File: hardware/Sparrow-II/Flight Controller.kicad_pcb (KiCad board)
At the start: 4 copper layers, 42 x 42 mm, 4 parts

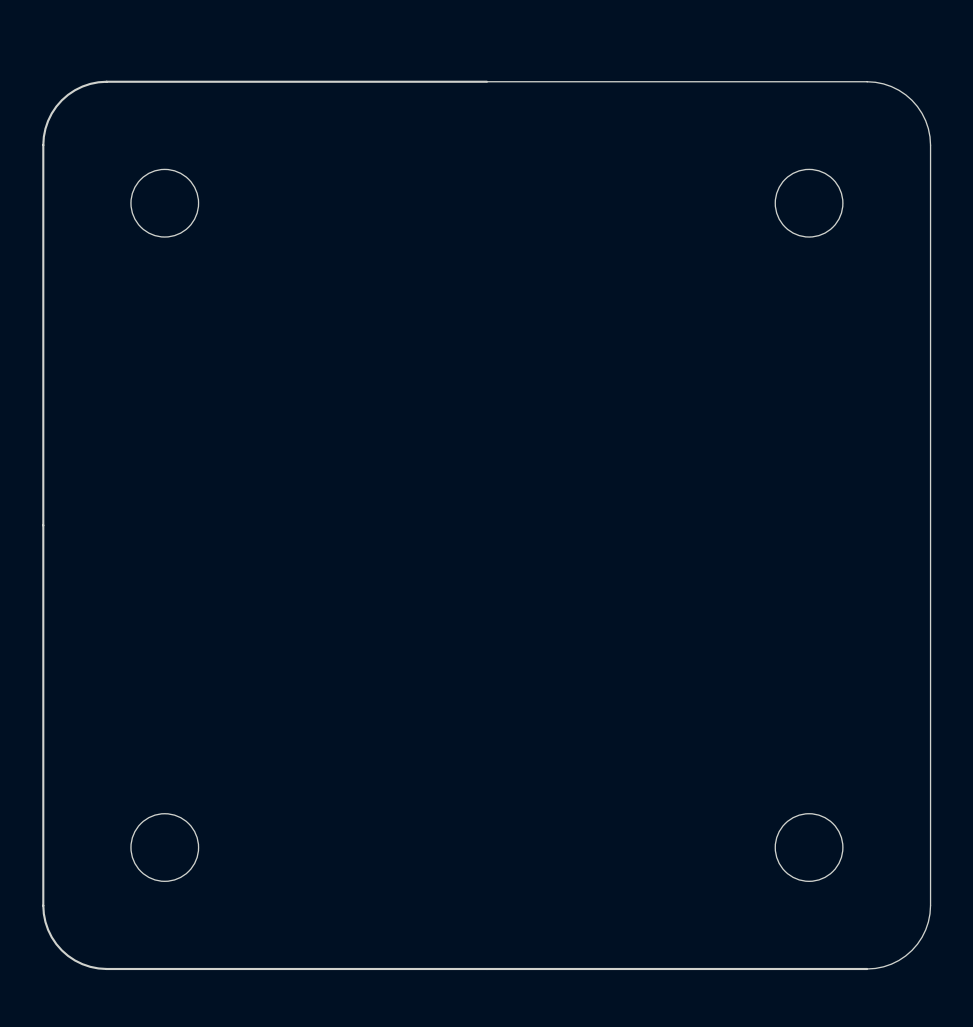
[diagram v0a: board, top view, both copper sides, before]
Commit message: hardware: first layout and optimalizations
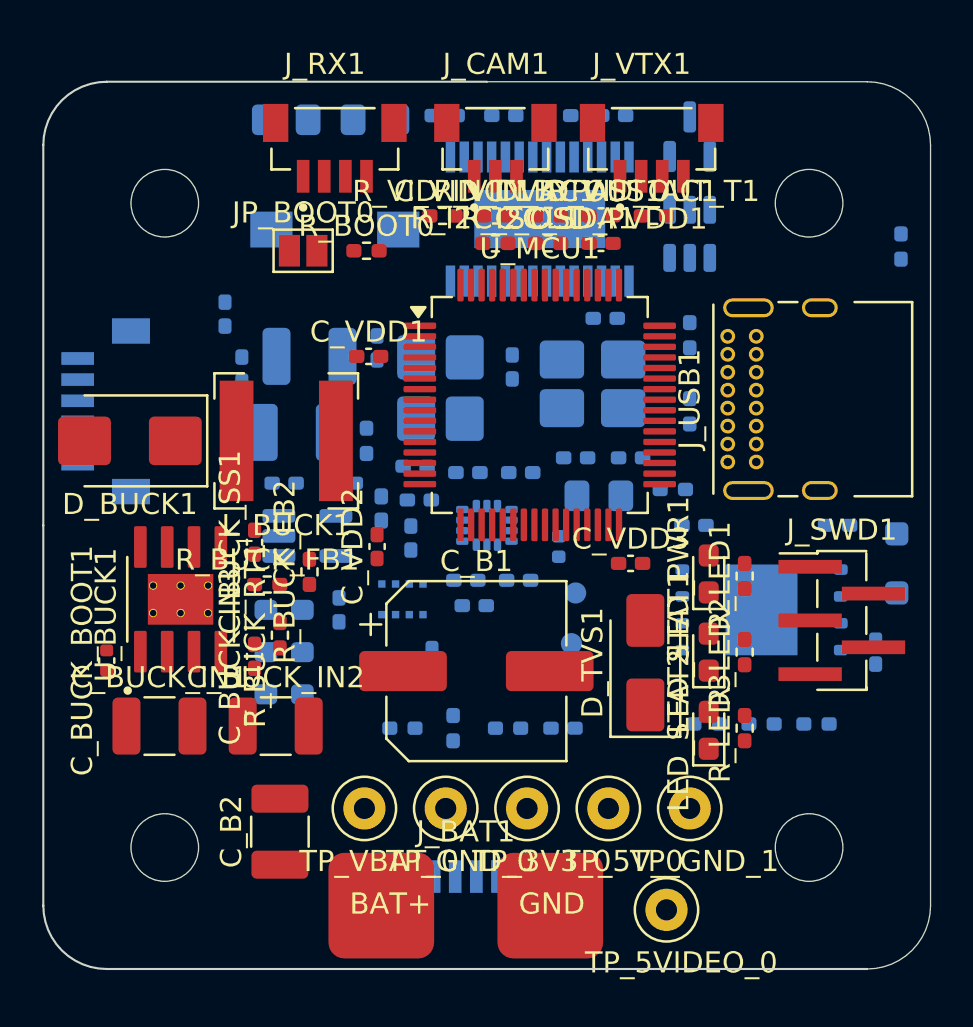
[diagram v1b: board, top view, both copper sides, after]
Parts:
- added C_3V3_BULK1: 10uF, Capacitor_SMD:C_0603_1608Metric_Pad1.08x0.95mm_HandSolder, B.Cu at (140.4, 104.0)
- added C_5V_BULK1: 10uF, Capacitor_SMD:C_0603_1608Metric_Pad1.08x0.95mm_HandSolder, B.Cu at (140.4, 108.0)
- added C_B1: 470uF, Capacitor_SMD:CP_Elec_8x6.9, F.Cu at (149.5, 106.9)
- added C_B2: 10uF, Capacitor_SMD:C_1210_3225Metric_Pad1.33x2.70mm_HandSolder, F.Cu at (140.2, 114.5)
- added C_B3: 1uF, Capacitor_SMD:C_0603_1608Metric_Pad1.08x0.95mm_HandSolder, B.Cu at (140.4, 106.0)
- added C_B4: 100nF, Capacitor_SMD:C_0402_1005Metric_Pad0.74x0.62mm_HandSolder, B.Cu at (143.0, 104.0)
- added C_BARO1: 100nF, Capacitor_SMD:C_0402_1005Metric_Pad0.74x0.62mm_HandSolder, B.Cu at (145.0, 106.4)
- added C_BARO2: 100nF, Capacitor_SMD:C_0402_1005Metric_Pad0.74x0.62mm_HandSolder, B.Cu at (147.4, 106.4)
- added C_BUCK_BOOT1: 100nF, Capacitor_SMD:C_0402_1005Metric, F.Cu at (132.0, 106.4)
- added C_BUCK_IN1: 2.2uF, Capacitor_SMD:C_1210_3225Metric_Pad1.33x2.70mm_HandSolder, F.Cu at (134.5, 109.5)
- added C_BUCK_IN2: 2.2uF, Capacitor_SMD:C_1210_3225Metric_Pad1.33x2.70mm_HandSolder, F.Cu at (140.0, 109.5)
- added C_BUCK_IN3: 100nF, Capacitor_SMD:C_0402_1005Metric_Pad0.74x0.62mm_HandSolder, F.Cu at (139.0, 106.2)
- added C_BUCK_OUT1: 47uF, Capacitor_SMD:C_1210_3225Metric_Pad1.33x2.70mm_HandSolder, B.Cu at (141.6, 92.0)
- added C_BUCK_OUT2: 47uF, Capacitor_SMD:C_1210_3225Metric_Pad1.33x2.70mm_HandSolder, B.Cu at (141.0, 95.6)
- added C_BUCK_SS1: 22nF, Capacitor_SMD:C_0402_1005Metric_Pad0.74x0.62mm_HandSolder, F.Cu at (139.0, 100.8)
- added C_CURR_F1: 1uF, Capacitor_SMD:C_0402_1005Metric_Pad0.74x0.62mm_HandSolder, B.Cu at (153.6, 109.6)
- added C_FLASH1: 100nF, Capacitor_SMD:C_0402_1005Metric_Pad0.74x0.62mm_HandSolder, B.Cu at (168.4, 106.0)
- added C_HSE1: 12pF, Capacitor_SMD:C_0402_1005Metric_Pad0.74x0.62mm_HandSolder, B.Cu at (146.6, 97.2)
- added C_HSE2: 12pF, Capacitor_SMD:C_0402_1005Metric_Pad0.74x0.62mm_HandSolder, B.Cu at (151.2, 92.5)
- added C_IMU_VDD1: 2.2uF, Capacitor_SMD:C_0402_1005Metric_Pad0.74x0.62mm_HandSolder, B.Cu at (151.5, 102.6)
- added C_IMU_VDD2: 100nF, Capacitor_SMD:C_0402_1005Metric_Pad0.74x0.62mm_HandSolder, B.Cu at (151.6, 97.5)
- added C_IMU_VIO1: 100nF, Capacitor_SMD:C_0402_1005Metric_Pad0.74x0.62mm_HandSolder, B.Cu at (149.1, 97.5)
- added C_IMU_VIO2: 10nF, Capacitor_SMD:C_0402_1005Metric_Pad0.74x0.62mm_HandSolder, B.Cu at (149.0, 102.6)
- added C_LDO_IN1: 1uF, Capacitor_SMD:C_0402_1005Metric_Pad0.74x0.62mm_HandSolder, B.Cu at (140.4, 98.0)
- added C_LDO_OUT1: 1uF, Capacitor_SMD:C_0402_1005Metric_Pad0.74x0.62mm_HandSolder, B.Cu at (143.2, 98.0)
- added C_NRST1: 100nF, Capacitor_SMD:C_0402_1005Metric_Pad0.74x0.62mm_HandSolder, B.Cu at (149.4, 103.8)
- added C_OSD_AVDD1: 100nF, Capacitor_SMD:C_0402_1005Metric_Pad0.74x0.62mm_HandSolder, B.Cu at (150.8, 80.6)
- added C_OSD_DVDD1: 100nF, Capacitor_SMD:C_0402_1005Metric_Pad0.74x0.62mm_HandSolder, B.Cu at (155.6, 90.2)
- added C_OSD_PVDD1: 4.7uF, Capacitor_SMD:C_0402_1005Metric_Pad0.74x0.62mm_HandSolder, F.Cu at (155.4, 86.7)
- added C_OSD_PVDD2: 100nF, Capacitor_SMD:C_0402_1005Metric_Pad0.74x0.62mm_HandSolder, B.Cu at (153.4, 80.6)
- added C_OSD_SAG1: 22uF, Capacitor_SMD:C_0402_1005Metric_Pad0.74x0.62mm_HandSolder, B.Cu at (156.0, 80.6)
- added C_OSD_XTAL1: 27pF, Capacitor_SMD:C_0402_1005Metric_Pad0.74x0.62mm_HandSolder, B.Cu at (154.2, 96.8)
- added C_OSD_XTAL2: 27pF, Capacitor_SMD:C_0402_1005Metric_Pad0.74x0.62mm_HandSolder, B.Cu at (156.8, 96.8)
- added C_USB_SH1: 10nF, Capacitor_SMD:C_0402_1005Metric_Pad0.74x0.62mm_HandSolder, B.Cu at (166.6, 100.0)
- added C_VBAT_ADC1: 100nF, Capacitor_SMD:C_0402_1005Metric_Pad0.74x0.62mm_HandSolder, B.Cu at (138.4, 92.6)
- added C_VCAP1: 4.7uF, Capacitor_SMD:C_0805_2012Metric_Pad1.18x1.45mm_HandSolder, B.Cu at (155.3, 98.6)
- added C_VDD1: 100nF, Capacitor_SMD:C_0402_1005Metric_Pad0.74x0.62mm_HandSolder, F.Cu at (144.4, 92.0)
- added C_VDD2: 100nF, Capacitor_SMD:C_0402_1005Metric_Pad0.74x0.62mm_HandSolder, F.Cu at (144.8, 101.0)
- added C_VDD3: 100nF, Capacitor_SMD:C_0402_1005Metric_Pad0.74x0.62mm_HandSolder, F.Cu at (156.8, 101.8)
- added C_VDD4: 100nF, Capacitor_SMD:C_0402_1005Metric_Pad0.74x0.62mm_HandSolder, B.Cu at (159.8, 100.0)
- added C_VDDA1: 1uF, Capacitor_SMD:C_0402_1005Metric_Pad0.74x0.62mm_HandSolder, B.Cu at (146.4, 100.6)
- added C_VDDA_HF1: 100nF, Capacitor_SMD:C_0402_1005Metric_Pad0.74x0.62mm_HandSolder, B.Cu at (146.8, 98.8)
- added C_VDD_BULK1: 4.7uF, Capacitor_SMD:C_0402_1005Metric_Pad0.74x0.62mm_HandSolder, B.Cu at (144.8, 91.6)
- added C_VID1: 22uF, Capacitor_SMD:C_0805_2012Metric_Pad1.18x1.45mm_HandSolder, B.Cu at (140.5, 80.8)
- added C_VID2: 22uF, Capacitor_SMD:C_0805_2012Metric_Pad1.18x1.45mm_HandSolder, B.Cu at (144.7, 80.8)
- added C_VID3: 100nF, Capacitor_SMD:C_0402_1005Metric_Pad0.74x0.62mm_HandSolder, B.Cu at (137.6, 90.0)
- added C_VID_IN_AC1: 100nF, Capacitor_SMD:C_0402_1005Metric_Pad0.74x0.62mm_HandSolder, F.Cu at (150.4, 85.3)
- added C_VID_OUT_AC1: 22uF, Capacitor_SMD:C_0402_1005Metric_Pad0.74x0.62mm_HandSolder, F.Cu at (155.4, 85.3)
- added D_BUCK1: B560C-13-F, Diode_SMD:D_SMB, F.Cu at (133.1, 96.0)
- added D_TVS1: SMAJ28A, Diode_SMD:D_SMA, F.Cu at (157.5, 106.5)
- added D_USB_VBUS1: PMEG2010AEH, Diode_SMD:D_SOD-123F, B.Cu at (169.4, 101.8)
- added D_VID_CLAMP1: BAV99, Package_TO_SOT_SMD:SOT-23, B.Cu at (159.6, 81.6)
- added FB_IMU1: 600R @ 100MHz, Inductor_SMD:L_0402_1005Metric, B.Cu at (153.4, 101.0)
- added FB_VDDA1: 100R @ 100MHz, Inductor_SMD:L_0402_1005Metric_Pad0.77x0.64mm_HandSolder, B.Cu at (145.0, 99.2)
- added JP_BOOT0: Jumper2, Jumper:SolderJumper-2_P1.3mm_Open_Pad1.0x1.5mm, F.Cu at (141.3, 87.0)
- added J_BAT1: Conn_01x02, SparrowHawk:VBAT_SolderPad_2x_5x5mm, F.Cu at (149.0, 118.0)
- added J_CAM1: BM03B-SRSS-TB_LF__SN_, SparrowHawk:JST_BM03B-SRSS-TB_LF__SN_, F.Cu at (150.4, 81.7)
- added J_ESC1: BM08B-SRSS-TB_LF__SN_, SparrowHawk:JST_BM08B-SRSS-TB_LF__SN_, B.Cu at (150.0, 118.4)
- added J_GPS1: BM06B-SRSS-TB_LF__SN_, SparrowHawk:JST_BM06B-SRSS-TB_LF__SN_, B.Cu at (132.4, 94.6)
- added J_RX1: BM04B-SRSS-TB_LF__SN_, SparrowHawk:JST_BM04B-SRSS-TB_LF__SN_, F.Cu at (142.8, 81.7)
- added J_SWD1: Conn_01x05, Connector_PinHeader_1.27mm:PinHeader_1x05_P1.27mm_Vertical_SMD_Pin1Left, F.Cu at (166.8, 104.5)
- added J_USB1: USB_C_Receptacle_USB2.0_16P, Connector_USB:USB_C_Receptacle_GCT_USB4085, F.Cu at (161.4, 97.0)
- added J_VTX1: BM04B-SRSS-TB_LF__SN_, SparrowHawk:JST_BM04B-SRSS-TB_LF__SN_, F.Cu at (157.8, 81.7)
- added LED_PWR1: LED Green 0603, LED_SMD:LED_0603_1608Metric_Pad1.05x0.95mm_HandSolder, F.Cu at (160.5, 102.3)
- added LED_STAT1: LED Blue 0603, LED_SMD:LED_0603_1608Metric_Pad1.05x0.95mm_HandSolder, F.Cu at (160.5, 106.0)
- added LED_STAT2: LED Red 0603, LED_SMD:LED_0603_1608Metric_Pad1.05x0.95mm_HandSolder, F.Cu at (160.5, 109.7)
- added L_BUCK1: 6.8uH, Inductor_SMD:L_Bourns-SRN6028, F.Cu at (140.5, 96.0)
- added L_VID1: 4.7uH, Inductor_SMD:L_Wuerth_WE-PD-Typ-7345, B.Cu at (142.8, 86.0)
- added R_BOOT0: 10k, Resistor_SMD:R_0402_1005Metric_Pad0.72x0.64mm_HandSolder, F.Cu at (144.3, 87.0)
- added R_BUCK_FB1: 100k, Resistor_SMD:R_0402_1005Metric_Pad0.72x0.64mm_HandSolder, F.Cu at (139.6, 102.8)
- added R_BUCK_FB2: 17.8k, Resistor_SMD:R_0402_1005Metric_Pad0.72x0.64mm_HandSolder, F.Cu at (141.6, 102.2)
- added R_BUCK_RT1: 49.9k, Resistor_SMD:R_0402_1005Metric_Pad0.72x0.64mm_HandSolder, F.Cu at (140.2, 105.2)
- added R_CC1: 5.1k, Resistor_SMD:R_0402_1005Metric_Pad0.72x0.64mm_HandSolder, B.Cu at (159.6, 91.0)
- added R_CC2: 5.1k, Resistor_SMD:R_0402_1005Metric_Pad0.72x0.64mm_HandSolder, B.Cu at (169.6, 86.8)
- added R_CURR_F1: 1k, Resistor_SMD:R_0402_1005Metric_Pad0.72x0.64mm_HandSolder, B.Cu at (151.0, 109.6)
- added R_FLASH_CS1: 10k, Resistor_SMD:R_0402_1005Metric_Pad0.72x0.64mm_HandSolder, B.Cu at (160.4, 109.4)
- added R_FLASH_HD1: 10k, Resistor_SMD:R_0402_1005Metric_Pad0.72x0.64mm_HandSolder, B.Cu at (165.6, 109.4)
- added R_FLASH_WP1: 10k, Resistor_SMD:R_0402_1005Metric_Pad0.72x0.64mm_HandSolder, B.Cu at (163.0, 109.4)
- added R_HSE1: 0R, Resistor_SMD:R_0402_1005Metric_Pad0.72x0.64mm_HandSolder, B.Cu at (158.8, 98.3)
- added R_HSE2: 0R, Resistor_SMD:R_0402_1005Metric_Pad0.72x0.64mm_HandSolder, B.Cu at (144.3, 96.0)
- added R_I2C_SCL1: 4.7k, Resistor_SMD:R_0402_1005Metric_Pad0.72x0.64mm_HandSolder, F.Cu at (150.4, 86.7)
- added R_I2C_SDA1: 4.7k, Resistor_SMD:R_0402_1005Metric_Pad0.72x0.64mm_HandSolder, F.Cu at (152.9, 86.7)
- added R_LED1: 1k, Resistor_SMD:R_0402_1005Metric_Pad0.72x0.64mm_HandSolder, F.Cu at (162.2, 102.4)
- added R_LED2: 1k, Resistor_SMD:R_0402_1005Metric_Pad0.72x0.64mm_HandSolder, F.Cu at (162.2, 106.0)
- added R_LED3: 1k, Resistor_SMD:R_0402_1005Metric_Pad0.72x0.64mm_HandSolder, F.Cu at (162.2, 109.6)
- added R_OSD_RST1: 10k, Resistor_SMD:R_0402_1005Metric_Pad0.72x0.64mm_HandSolder, B.Cu at (148.0, 80.6)
- added R_USB_SH1: 1M, Resistor_SMD:R_0402_1005Metric_Pad0.72x0.64mm_HandSolder, B.Cu at (159.6, 94.6)
- added R_VBAT_D1: 100k, Resistor_SMD:R_0402_1005Metric_Pad0.72x0.64mm_HandSolder, B.Cu at (146.0, 109.6)
- added R_VBAT_D2: 10k, Resistor_SMD:R_0402_1005Metric_Pad0.72x0.64mm_HandSolder, B.Cu at (148.4, 109.6)
- added R_VID_BYPASS1: 0R, Resistor_SMD:R_0402_1005Metric_Pad0.72x0.64mm_HandSolder, F.Cu at (152.9, 85.3)
- added R_VID_IN_T1: 75R, Resistor_SMD:R_0402_1005Metric_Pad0.72x0.64mm_HandSolder, F.Cu at (147.9, 85.3)
- added R_VID_OUT_T1: 75R, Resistor_SMD:R_0402_1005Metric_Pad0.72x0.64mm_HandSolder, F.Cu at (157.9, 85.3)
- added TP_3V3_0: Test Point Loop, TestPoint:TestPoint_Loop_D1.80mm_Drill1.0mm_Beaded, F.Cu at (151.9, 113.4)
- added TP_5VIDEO_0: Test Point Loop, TestPoint:TestPoint_Loop_D1.80mm_Drill1.0mm_Beaded, F.Cu at (158.5, 118.2)
- added TP_5V_0: Test Point Loop, TestPoint:TestPoint_Loop_D1.80mm_Drill1.0mm_Beaded, F.Cu at (155.8, 113.4)
- added TP_GND_0: Test Point Loop, TestPoint:TestPoint_Loop_D1.80mm_Drill1.0mm_Beaded, F.Cu at (148.1, 113.4)
- added TP_GND_1: Test Point Loop, TestPoint:TestPoint_Loop_D1.80mm_Drill1.0mm_Beaded, F.Cu at (159.6, 113.4)
- added TP_IMU_INT_0: Test Point, TestPoint:TestPoint_Pad_D1.0mm, B.Cu at (154.2, 103.2)
- added TP_VBAT_0: Test Point Loop, TestPoint:TestPoint_Loop_D1.80mm_Drill1.0mm_Beaded, F.Cu at (144.2, 113.4)
- added TP_VBAT_ADC_0: Test Point, TestPoint:TestPoint_Pad_D1.0mm, B.Cu at (154.0, 105.6)
- added U_BARO1: DPS310, SparrowHawk:XDCR_DPS310, B.Cu at (146.0, 103.5)
- added U_BUCK1: LMR14030SDDAR, SparrowHawk:SOIC127P600X170-9N, F.Cu at (135.5, 103.5)
- added U_ESD1: USBLC6-2SC6, Package_TO_SOT_SMD:SOT-23-6, B.Cu at (159.6, 86.2)
- added U_FLASH1: W25Q128JVE, Package_SON:WSON-8-1EP_8x6mm_P1.27mm_EP3.4x4.3mm, B.Cu at (163.0, 104.0)
- added U_IMU1: ICM-42688-P, SparrowHawk:PQFN50P300X250X97-14N, B.Cu at (150.0, 100.0)
- added U_LDO1: AP2112K-3.3TRG1, Package_TO_SOT_SMD:SOT-23-5_HandSoldering, B.Cu at (141.5, 100.5)
- added U_MCU1: STM32F722RETx, Package_QFP:LQFP-64_10x10mm_P0.5mm, F.Cu at (152.5, 94.3)
- added U_OSD1: AT7456E, SparrowHawk:SOP65P640X120-29N, B.Cu at (152.5, 85.5)
- added Y_HSE1: 8MHz CL=10pF ESR<150R, Crystal:Crystal_SMD_3225-4Pin_3.2x2.5mm_HandSoldering, B.Cu at (147.8, 93.5)
- added Y_OSD1: 27MHz, Crystal:Crystal_SMD_3225-4Pin_3.2x2.5mm_HandSoldering, B.Cu at (155.0, 93.3)
